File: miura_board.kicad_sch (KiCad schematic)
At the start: 41 parts, among them J1 Screw_Terminal_01x02, J2 Screw_Terminal_01x02, J3 Screw_Terminal_01x02, J4 Conn_01x04_Male, J5 Screw_Terminal_01x02, J6 Screw_Terminal_01x02, J7 Screw_Terminal_01x02, J8 Screw_Terminal_01x02, SW1 SW_Push, SW2 SW_Push, U1 ESP32-WROOM, U2 W25Q32JVSS, U3 DRV8833PW, U4 DRV8833PW, U5 AMS1117, U6 MPU-6050, U7 L7806, U8 DRV8833PW

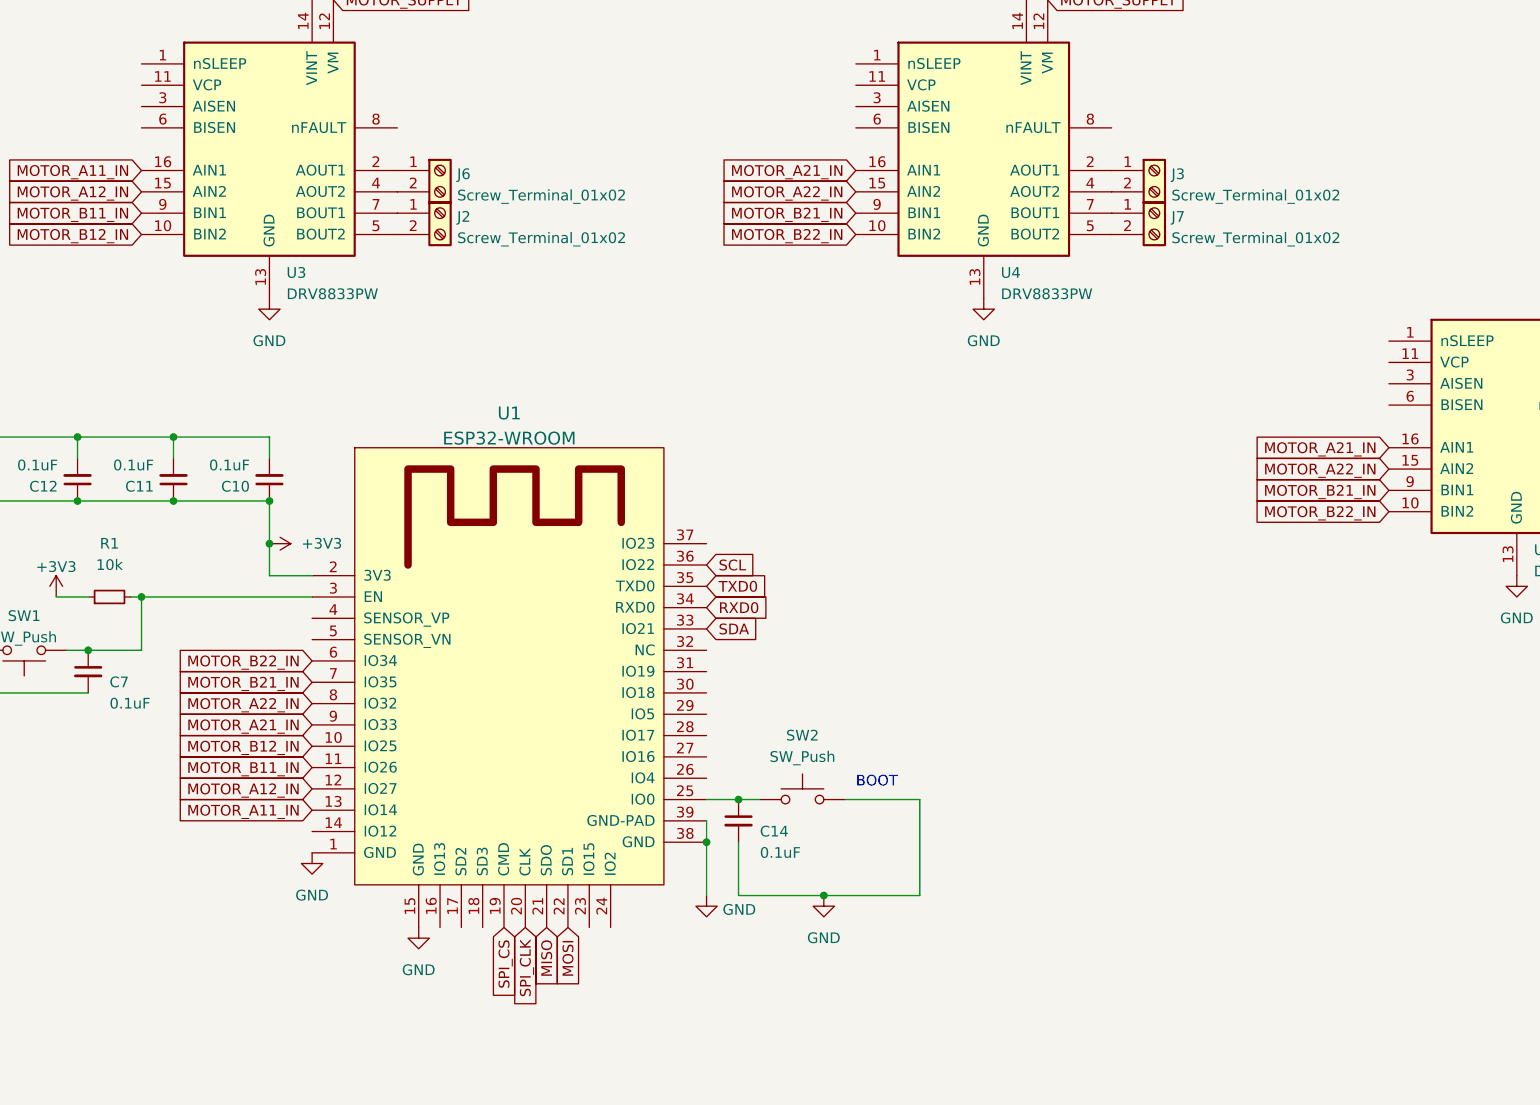
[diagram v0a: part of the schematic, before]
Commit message: lol
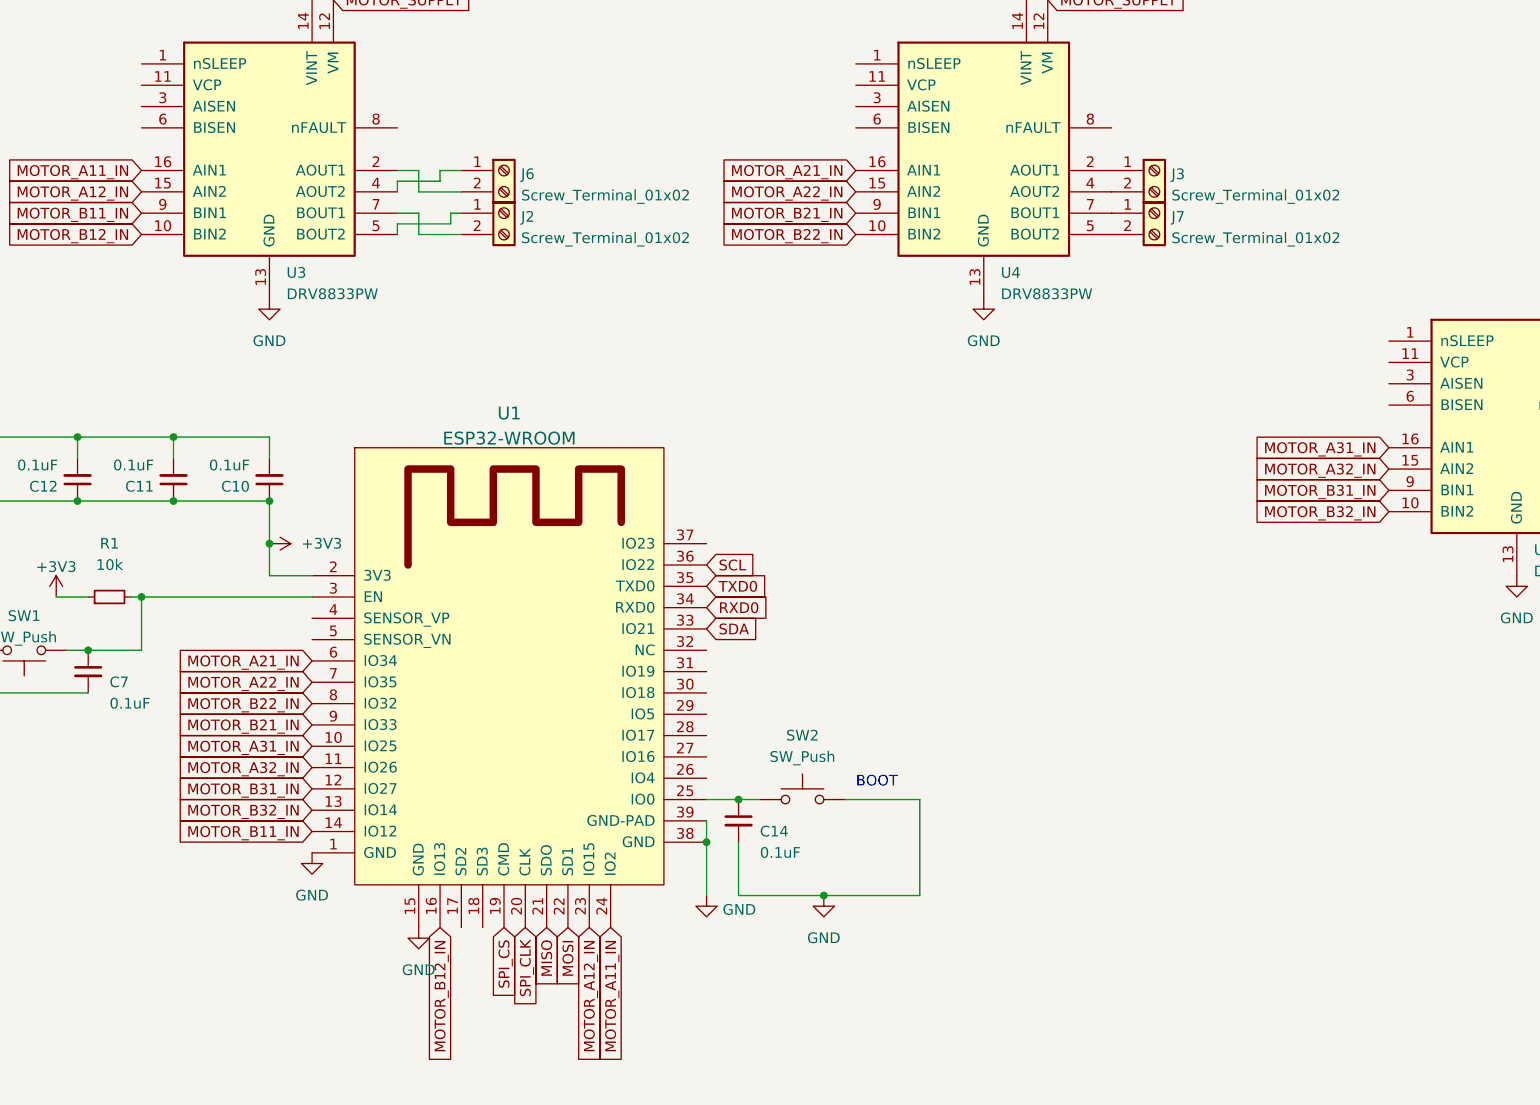
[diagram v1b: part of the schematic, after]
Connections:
- net MOTOR_A11_IN: now also U1.24 (IO2); no longer U1.13 (IO14)
- net MOTOR_A12_IN: now also U1.23 (IO15); no longer U1.12 (IO27)
- net MOTOR_A21_IN: now also U1.6 (IO34); no longer U1.9 (IO33), U8.16 (AIN1)
- net MOTOR_A22_IN: now also U1.7 (IO35); no longer U1.8 (IO32), U8.15 (AIN2)
- net MOTOR_B11_IN: now also U1.14 (IO12); no longer U1.11 (IO26)
- net MOTOR_B12_IN: now also U1.16 (IO13); no longer U1.10 (IO25)
- net MOTOR_B21_IN: now also U1.9 (IO33); no longer U1.7 (IO35), U8.9 (BIN1)
- net MOTOR_B22_IN: now also U1.8 (IO32); no longer U1.6 (IO34), U8.10 (BIN2)
- net at U3.2 (AOUT1): now also J6.2 (Pin_2); no longer J6.1 (Pin_1)
- net at U3.4 (AOUT2): now also J6.1 (Pin_1); no longer J6.2 (Pin_2)
- net at U3.5 (BOUT2): now also J2.1 (Pin_1); no longer J2.2 (Pin_2)
- net at U3.7 (BOUT1): now also J2.2 (Pin_2); no longer J2.1 (Pin_1)
- new net MOTOR_A31_IN: U1.10 (IO25), U8.16 (AIN1)
- new net MOTOR_A32_IN: U1.11 (IO26), U8.15 (AIN2)
- new net MOTOR_B31_IN: U1.12 (IO27), U8.9 (BIN1)
- new net MOTOR_B32_IN: U1.13 (IO14), U8.10 (BIN2)
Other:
- moved on the sheet: J2, J6
